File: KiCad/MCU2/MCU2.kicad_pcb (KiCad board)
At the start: 2 copper layers, 47.6 x 37.1 mm, 16 parts, among them J1 Conn_02x03_Counter_Clockwise, J2 Conn_01x06, J3 Conn_01x03, J4 Conn_01x02_Pin, J5 XT30, J6 AandDpin, SW1 MCU_Button, U1 ATmega328P-A, U2 AMS1117, U3 ADR02AUJZ-REEL7

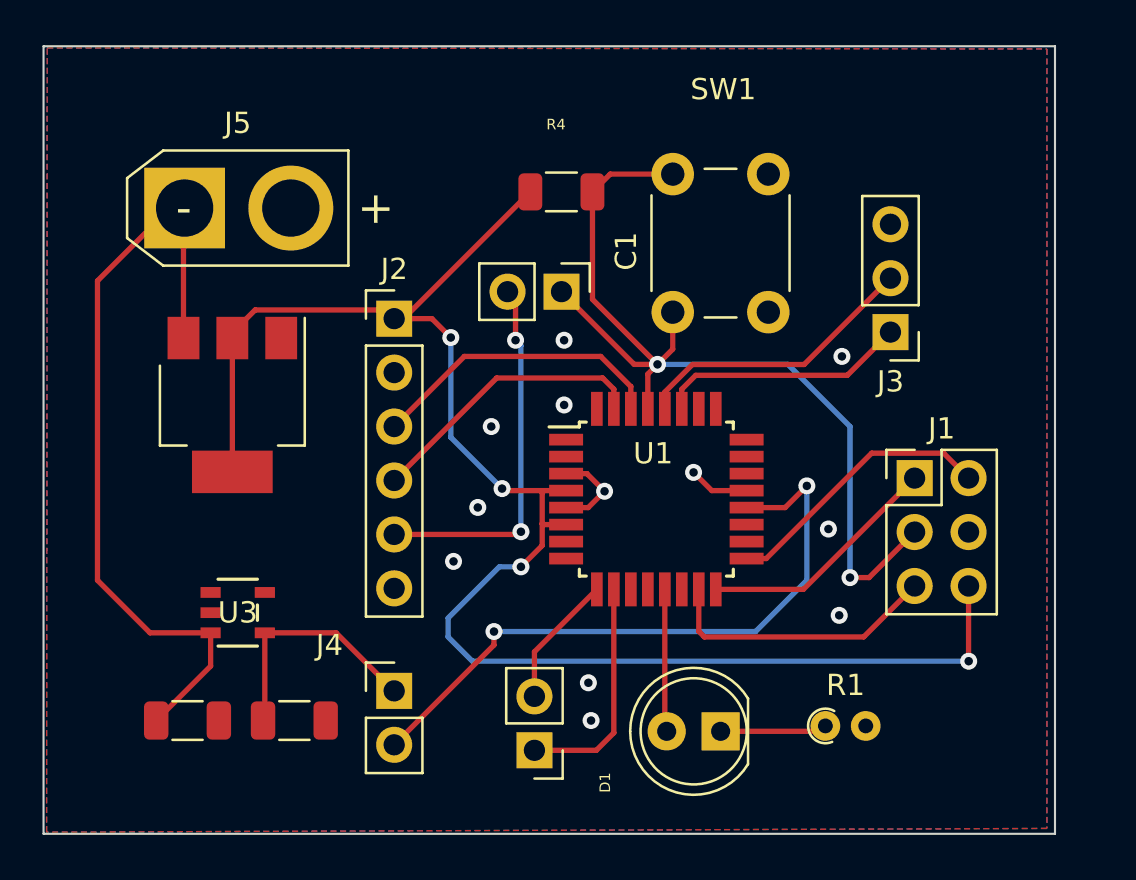
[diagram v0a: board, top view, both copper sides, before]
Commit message: update
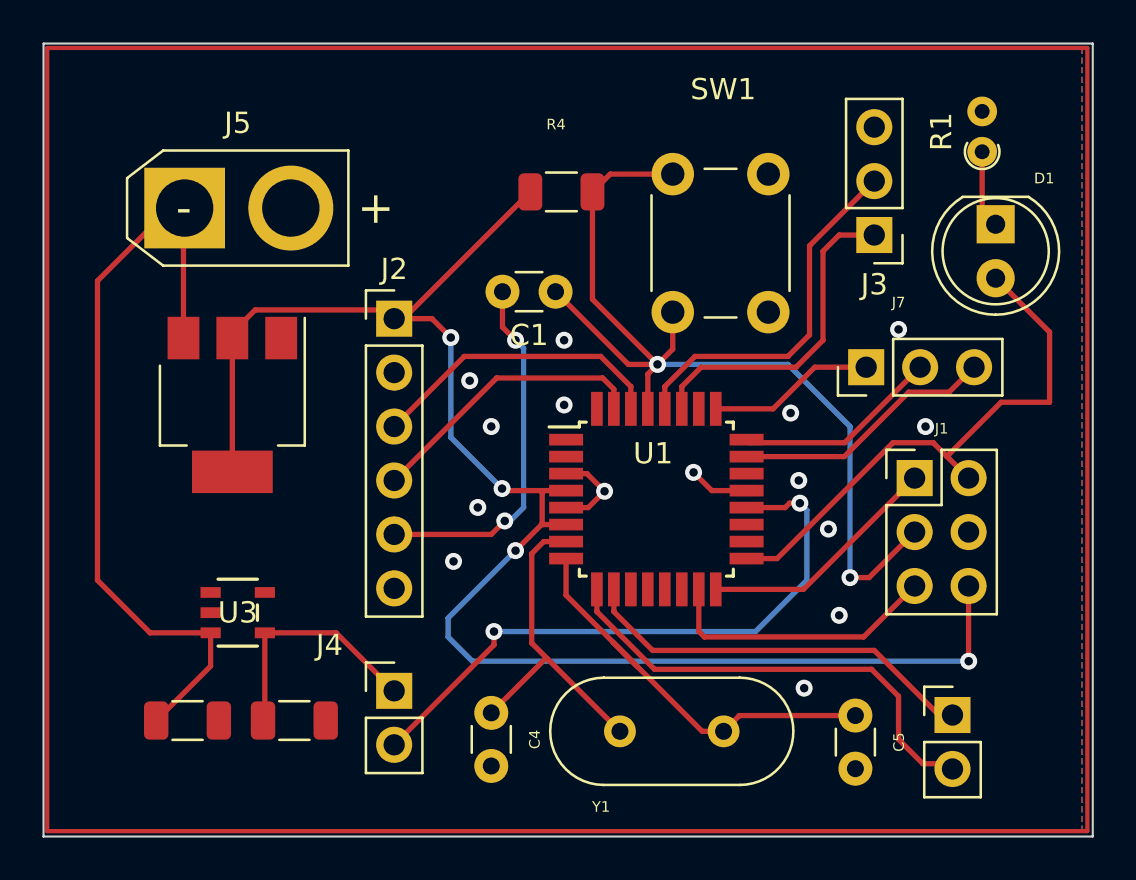
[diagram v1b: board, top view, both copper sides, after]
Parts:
- added C4: 0.22pf, Capacitor_THT:C_Disc_D3.0mm_W1.6mm_P2.50mm, F.Cu at (122.6, 85.9)
- added C5: 0.22pf, Capacitor_THT:C_Disc_D3.0mm_W1.6mm_P2.50mm, F.Cu at (139.7, 86.0)
- added J7: Conn_01x03, Connector_PinHeader_2.54mm:PinHeader_1x03_P2.54mm_Vertical, F.Cu at (140.2, 69.6)
- added Y1: Crystal, Crystal:Crystal_HC49-4H_Vertical, F.Cu at (128.6, 86.7)
- C1: footprint Connector_PinHeader_2.54mm:PinHeader_1x02_P2.54mm_Vertical -> Capacitor_THT:C_Disc_D3.0mm_W1.6mm_P2.50mm
- moved R1 28.0 mm to (145.7, 59.5), turned to 90 degrees
- moved D1 27.2 mm to (146.3, 62.9), turned to -90 degrees
- moved J6 19.8 mm to (144.3, 86.0), turned to 0 degrees
- moved J3 4.64 mm to (140.6, 63.4)
- moved C1 0.28 mm to (125.6, 66.0), turned to 180 degrees
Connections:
- D1 pad 2: Net-(D1-A) -> /SCK
- U1 pad 13: Net-(D1-A) -> unconnected-(U1-PB1-Pad13)
- U1 pad 23: unconnected-(U1-PC0-Pad23) -> Net-(J7-Pin_3)
- U1 pad 24: unconnected-(U1-PC1-Pad24) -> Net-(J7-Pin_2)
- U1 pad 25: unconnected-(U1-PC2-Pad25) -> Net-(J7-Pin_1)
- U1 pad 7: unconnected-(U1-XTAL1/PB6-Pad7) -> Net-(U1-XTAL1/PB6)
- U1 pad 8: unconnected-(U1-XTAL2/PB7-Pad8) -> Net-(U1-XTAL2/PB7)
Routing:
- net Net-(U1-XTAL2/PB7): track 0.00 -> 19.9 mm
- net /Digital: track 6.26 -> 22.1 mm
- net Net-(U1-XTAL1/PB6): track 0.00 -> 15.6 mm
- net /SCK: track 13.0 -> 26.2 mm
- net Net-(J7-Pin_3): track 0.00 -> 12.5 mm
- net Net-(J7-Pin_2): track 0.00 -> 9.70 mm
- net /Analog: track 10.8 -> 19.0 mm
- net Net-(J7-Pin_1): track 0.00 -> 7.89 mm
- net Net-(D1-A): track 6.72 -> 0.00 mm
- net /SCL: track 13.6 -> 17.4 mm
- net /SDA: track 11.9 -> 15.5 mm
- net Net-(D1-K): track 5.04 -> 3.68 mm
- net /AREF: track 30.7 -> 29.4 mm
- net +5V: track 76.9 -> 76.3 mm
- net GND: vias 12 -> 15
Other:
- board size 47.6 x 37.1 mm -> 49.4 x 37.3 mm
- board text added: "烨"
